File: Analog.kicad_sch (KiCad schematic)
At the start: 20 parts, among them U3 74HC4051, U4 74HC4051, U5 OPA350

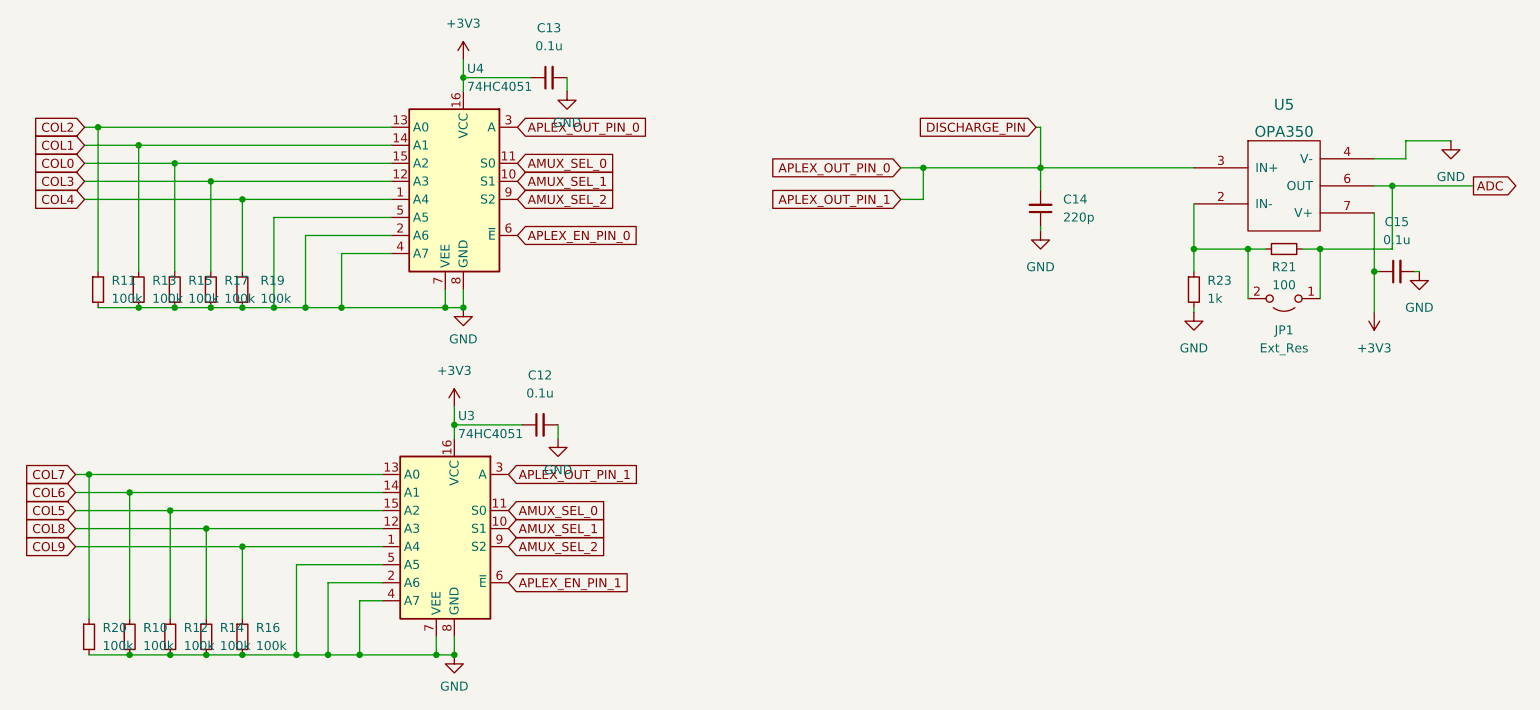
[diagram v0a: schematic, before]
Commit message: production files
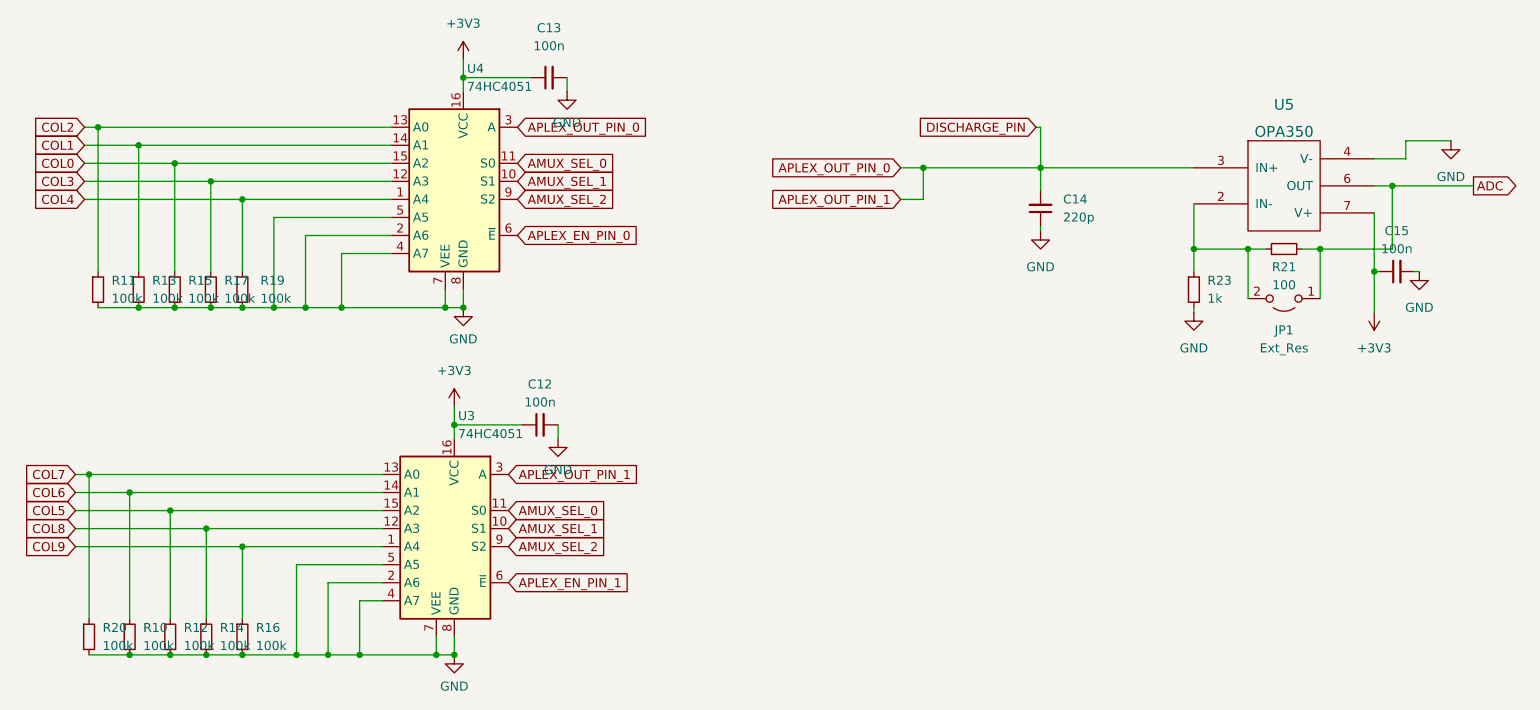
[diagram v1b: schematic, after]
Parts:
- C12, C13, C15: value 0.1u -> 100n
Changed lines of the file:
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@@
     (pin "2")
     (instances
-      (project "travaulta rgb"
+      (project "travaulta"
         (path "/690df46b-b605-4617-b545-6aaced86d0fc/197f4772-e814-41eb-a239-e401e14c7029"
           (reference "C14") (unit 1)
@@
     (pin "2")
     (instances
-      (project "travaulta rgb"
+      (project "travaulta"
         (path "/690df46b-b605-4617-b545-6aaced86d0fc/197f4772-e814-41eb-a239-e401e14c7029"
           (reference "R20") (unit 1)
@@
     (pin "1")
     (instances
-      (project "travaulta rgb"
+      (project "travaulta"
         (path "/690df46b-b605-4617-b545-6aaced86d0fc/197f4772-e814-41eb-a239-e401e14c7029"
           (reference "#PWR0138") (unit 1)
@@
   (symbol (lib_id "Device:C_Small") (at 252.73 62.865 90) (unit 1)
     (in_bom yes) (on_board yes) (dnp no) (fields_autoplaced)
-    (property "Reference" "C15" (at 252.7363 55.88 90)
-      (effects (font (size 1.27 1.27)))
-    )
-    (property "Value" "0.1u" (at 252.7363 58.42 90)
+    (property "Reference" "C15" (at 252.7363 57.15 90)
+      (effects (font (size 1.27 1.27)))
+    )
+    (property "Value" "100n" (at 252.7363 59.69 90)
       (effects (font (size 1.27 1.27)))
     )
@@
     (pin "2")
     (instances
-      (project "travaulta rgb"
+      (project "travaulta"
         (path "/690df46b-b605-4617-b545-6aaced86d0fc/197f4772-e814-41eb-a239-e401e14c7029"
           (reference "C15") (unit 1)
@@
     (pin "7")
     (instances
-      (project "travaulta rgb"
+      (project "travaulta"
         (path "/690df46b-b605-4617-b545-6aaced86d0fc/197f4772-e814-41eb-a239-e401e14c7029"
           (reference "U5") (unit 1)
@@
     (pin "1")
     (instances
-      (project "travaulta rgb"
+      (project "travaulta"
         (path "/690df46b-b605-4617-b545-6aaced86d0fc/197f4772-e814-41eb-a239-e401e14c7029"
           (reference "#PWR0140") (unit 1)
@@
     (pin "9")
     (instances
-      (project "travaulta rgb"
+      (project "travaulta"
         (path "/690df46b-b605-4617-b545-6aaced86d0fc/197f4772-e814-41eb-a239-e401e14c7029"
           (reference "U3") (unit 1)
@@
     (pin "1")
     (instances
-      (project "travaulta rgb"
+      (project "travaulta"
         (path "/690df46b-b605-4617-b545-6aaced86d0fc/197f4772-e814-41eb-a239-e401e14c7029"
           (reference "#PWR0141") (unit 1)
@@
   (symbol (lib_id "Device:C_Small") (at 132.08 84.455 90) (unit 1)
     (in_bom yes) (on_board yes) (dnp no) (fields_autoplaced)
-    (property "Reference" "C12" (at 132.0863 77.47 90)
-      (effects (font (size 1.27 1.27)))
-    )
-    (property "Value" "0.1u" (at 132.0863 80.01 90)
+    (property "Reference" "C12" (at 132.0863 78.74 90)
+      (effects (font (size 1.27 1.27)))
+    )
+    (property "Value" "100n" (at 132.0863 81.28 90)
       (effects (font (size 1.27 1.27)))
     )
@@
     (pin "2")
     (instances
-      (project "travaulta rgb"
+      (project "travaulta"
         (path "/690df46b-b605-4617-b545-6aaced86d0fc/197f4772-e814-41eb-a239-e401e14c7029"
           (reference "C12") (unit 1)
@@
     (pin "2")
     (instances
-      (project "travaulta rgb"
+      (project "travaulta"
         (path "/690df46b-b605-4617-b545-6aaced86d0fc/197f4772-e814-41eb-a239-e401e14c7029"
           (reference "R10") (unit 1)
@@
     (pin "2")
     (instances
-      (project "travaulta rgb"
+      (project "travaulta"
         (path "/690df46b-b605-4617-b545-6aaced86d0fc/197f4772-e814-41eb-a239-e401e14c7029"
           (reference "R15") (unit 1)
@@
     (pin "2")
     (instances
-      (project "travaulta rgb"
+      (project "travaulta"
         (path "/690df46b-b605-4617-b545-6aaced86d0fc/197f4772-e814-41eb-a239-e401e14c7029"
           (reference "R11") (unit 1)
@@
     (pin "2")
     (instances
-      (project "travaulta rgb"
+      (project "travaulta"
         (path "/690df46b-b605-4617-b545-6aaced86d0fc/197f4772-e814-41eb-a239-e401e14c7029"
           (reference "R14") (unit 1)
@@
     (pin "1")
     (instances
-      (project "travaulta rgb"
+      (project "travaulta"
         (path "/690df46b-b605-4617-b545-6aaced86d0fc/197f4772-e814-41eb-a239-e401e14c7029"
           (reference "#PWR0136") (unit 1)
@@
     (pin "1")
     (instances
-      (project "travaulta rgb"
+      (project "travaulta"
         (path "/690df46b-b605-4617-b545-6aaced86d0fc/197f4772-e814-41eb-a239-e401e14c7029"
           (reference "#PWR0143") (unit 1)
@@
     (pin "9")
     (instances
-      (project "travaulta rgb"
+      (project "travaulta"
         (path "/690df46b-b605-4617-b545-6aaced86d0fc/197f4772-e814-41eb-a239-e401e14c7029"
           (reference "U4") (unit 1)
@@
     (pin "2")
     (instances
-      (project "travaulta rgb"
+      (project "travaulta"
         (path "/690df46b-b605-4617-b545-6aaced86d0fc/197f4772-e814-41eb-a239-e401e14c7029"
           (reference "R23") (unit 1)
@@
     (pin "1")
     (instances
-      (project "travaulta rgb"
+      (project "travaulta"
         (path "/690df46b-b605-4617-b545-6aaced86d0fc/197f4772-e814-41eb-a239-e401e14c7029"
           (reference "#PWR0148") (unit 1)
@@
     (pin "1")
     (instances
-      (project "travaulta rgb"
+      (project "travaulta"
         (path "/690df46b-b605-4617-b545-6aaced86d0fc/197f4772-e814-41eb-a239-e401e14c7029"
           (reference "#PWR0139") (unit 1)
@@
       (effects (font (size 1.27 1.27)))
     )
-    (property "Value" "0.1u" (at 133.3563 31.115 90)
+    (property "Value" "100n" (at 133.3563 31.115 90)
       (effects (font (size 1.27 1.27)))
     )
@@
     (pin "2")
     (instances
-      (project "travaulta rgb"
+      (project "travaulta"
         (path "/690df46b-b605-4617-b545-6aaced86d0fc/197f4772-e814-41eb-a239-e401e14c7029"
           (reference "C13") (unit 1)
@@
     (pin "2")
     (instances
-      (project "travaulta rgb"
+      (project "travaulta"
         (path "/690df46b-b605-4617-b545-6aaced86d0fc/197f4772-e814-41eb-a239-e401e14c7029"
           (reference "R21") (unit 1)
@@
     (pin "2")
     (instances
-      (project "travaulta rgb"
+      (project "travaulta"
         (path "/690df46b-b605-4617-b545-6aaced86d0fc/197f4772-e814-41eb-a239-e401e14c7029"
           (reference "R16") (unit 1)
@@
     (pin "2")
     (instances
-      (project "travaulta rgb"
+      (project "travaulta"
         (path "/690df46b-b605-4617-b545-6aaced86d0fc/197f4772-e814-41eb-a239-e401e14c7029"
           (reference "R17") (unit 1)
@@
     (pin "2")
     (instances
-      (project "travaulta rgb"
+      (project "travaulta"
         (path "/690df46b-b605-4617-b545-6aaced86d0fc/197f4772-e814-41eb-a239-e401e14c7029"
           (reference "R12") (unit 1)
@@
     (pin "2")
     (instances
-      (project "travaulta rgb"
+      (project "travaulta"
         (path "/690df46b-b605-4617-b545-6aaced86d0fc/197f4772-e814-41eb-a239-e401e14c7029"
           (reference "JP1") (unit 1)
@@
     (pin "1")
     (instances
-      (project "travaulta rgb"
+      (project "travaulta"
         (path "/690df46b-b605-4617-b545-6aaced86d0fc/197f4772-e814-41eb-a239-e401e14c7029"
           (reference "#PWR0135") (unit 1)
@@
     (pin "1")
     (instances
-      (project "travaulta rgb"
+      (project "travaulta"
         (path "/690df46b-b605-4617-b545-6aaced86d0fc/197f4772-e814-41eb-a239-e401e14c7029"
           (reference "#PWR0134") (unit 1)
@@
     (pin "1")
     (instances
-      (project "travaulta rgb"
+      (project "travaulta"
         (path "/690df46b-b605-4617-b545-6aaced86d0fc/197f4772-e814-41eb-a239-e401e14c7029"
           (reference "#PWR0142") (unit 1)
@@
     (pin "2")
     (instances
-      (project "travaulta rgb"
+      (project "travaulta"
         (path "/690df46b-b605-4617-b545-6aaced86d0fc/197f4772-e814-41eb-a239-e401e14c7029"
           (reference "R19") (unit 1)
@@
     (pin "1")
     (instances
-      (project "travaulta rgb"
+      (project "travaulta"
         (path "/690df46b-b605-4617-b545-6aaced86d0fc/197f4772-e814-41eb-a239-e401e14c7029"
           (reference "#PWR0137") (unit 1)
@@
     (pin "2")
     (instances
-      (project "travaulta rgb"
+      (project "travaulta"
         (path "/690df46b-b605-4617-b545-6aaced86d0fc/197f4772-e814-41eb-a239-e401e14c7029"
           (reference "R13") (unit 1)
